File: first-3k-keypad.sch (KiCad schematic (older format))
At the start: 14 parts

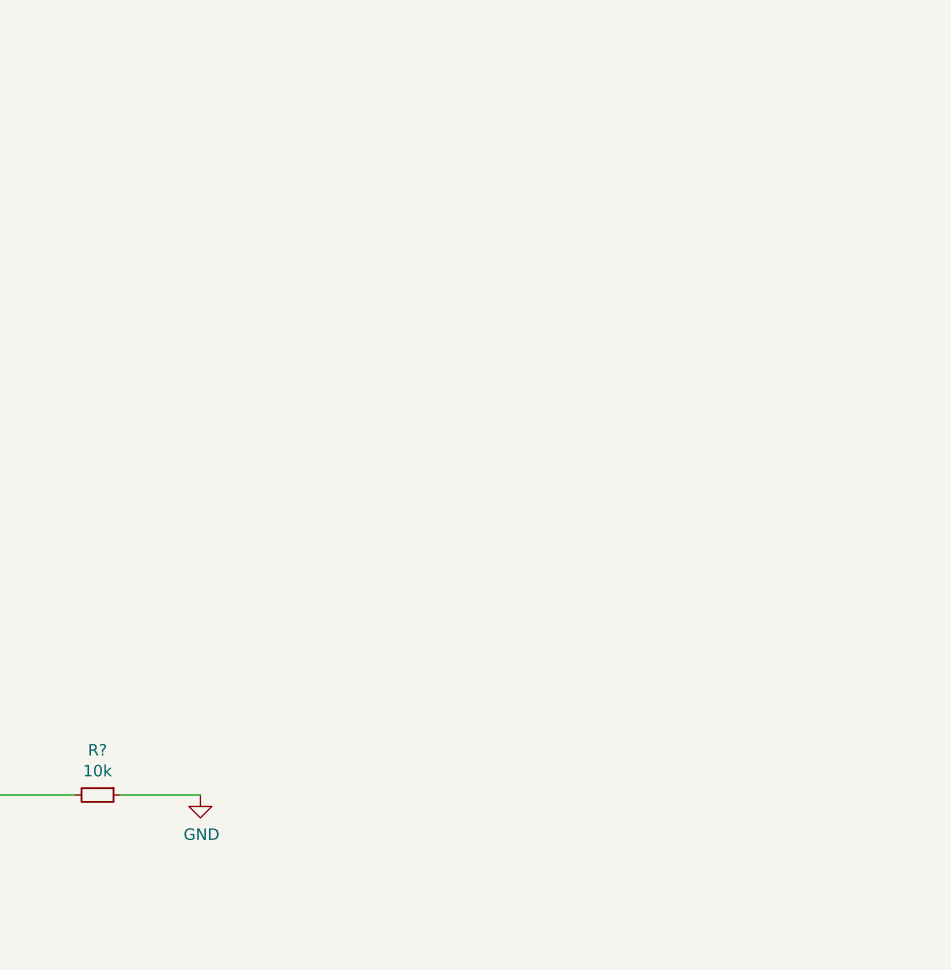
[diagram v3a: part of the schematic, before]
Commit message: Finished Schematic
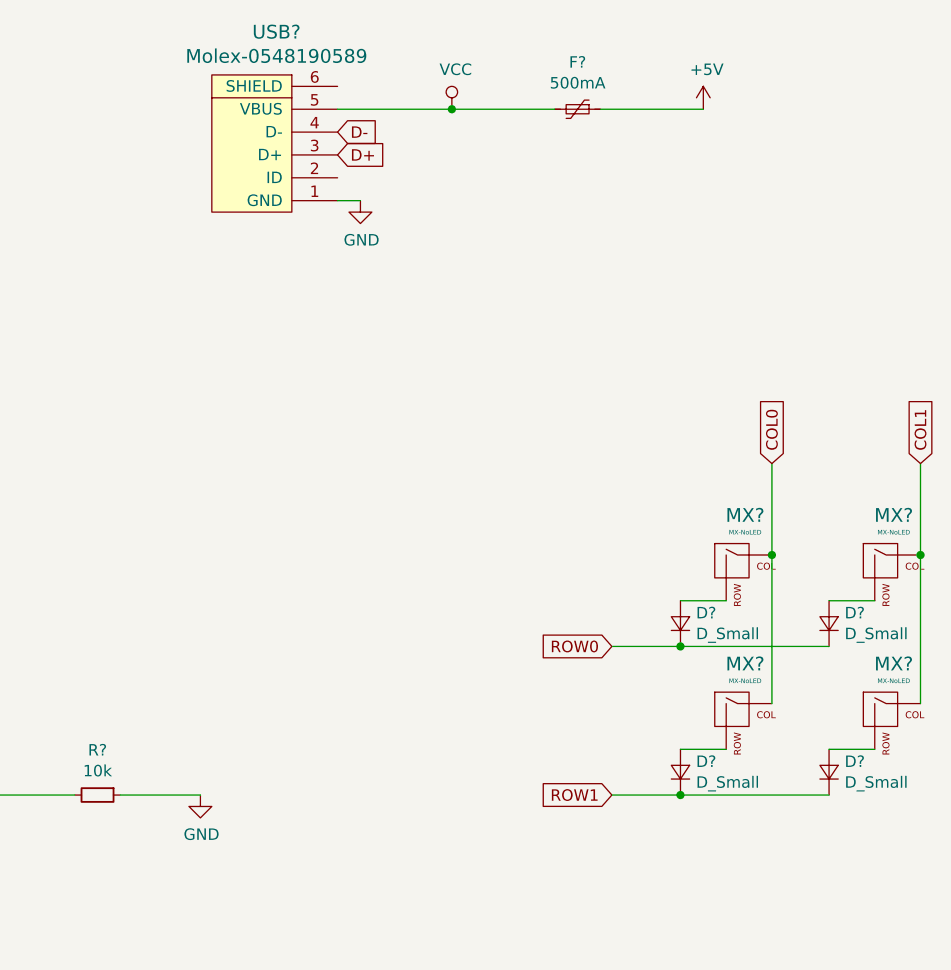
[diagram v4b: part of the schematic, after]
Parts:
- added D? (x4): D_Small, symbol Device:D_Small
- added F?: 500mA, symbol Device:Polyfuse_Small
- added MX? (x4): MX-NoLED, symbol MX_Alps_Hybrid:MX-NoLED
- added USB?: Molex-0548190589, symbol random-keyboard-parts:Molex-0548190589
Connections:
- net +5V: now also F?.1
- net D+: now also USB?.3 (D+)
- net D-: now also USB?.4 (D-)
- net GND: now also USB?.1 (GND)
- new net: D?.2 (A), MX?.2 (ROW) (x4)
- new net COL0: MX?.1 (COL), MX?.1 (COL)
- new net COL1: MX?.1 (COL), MX?.1 (COL)
- new net ROW0: D?.1 (K), D?.1 (K)
- new net ROW1: D?.1 (K), D?.1 (K)
- new net VCC: F?.2, USB?.5 (VBUS)
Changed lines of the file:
@@
 Text GLabel 4000 3500 0    50   Input ~ 0
 D-
+$Comp
+L random-keyboard-parts:Molex-0548190589 USB?
+U 1 1 6353D7B6
+P 7900 1700
+F 0 "USB?" V 8437 1667 60  0000 C CNN
+F 1 "Molex-0548190589" V 8331 1667 60  0000 C CNN
+F 2 "" H 7900 1700 60  0001 C CNN
+F 3 "" H 7900 1700 60  0001 C CNN
+	1    7900 1700
+	0    -1   -1   0
+$EndComp
+$Comp
+L Device:Polyfuse_Small F?
+U 1 1 6353F2F1
+P 9250 1500
+F 0 "F?" V 9045 1500 50  0000 C CNN
+F 1 "500mA" V 9136 1500 50  0000 C CNN
+F 2 "" H 9300 1300 50  0001 L CNN
+F 3 "~" H 9250 1500 50  0001 C CNN
+	1    9250 1500
+	0    1    1    0
+$EndComp
+$Comp
+L power:+5V #PWR?
+U 1 1 63542566
+P 9800 1500
+F 0 "#PWR?" H 9800 1350 50  0001 C CNN
+F 1 "+5V" H 9815 1673 50  0000 C CNN
+F 2 "" H 9800 1500 50  0001 C CNN
+F 3 "" H 9800 1500 50  0001 C CNN
+	1    9800 1500
+	1    0    0    -1
+$EndComp
+Wire Wire Line
+	9800 1500 9350 1500
+$Comp
+L power:VCC #PWR?
+U 1 1 63543A2B
+P 8700 1500
+F 0 "#PWR?" H 8700 1350 50  0001 C CNN
+F 1 "VCC" H 8717 1673 50  0000 C CNN
+F 2 "" H 8700 1500 50  0001 C CNN
+F 3 "" H 8700 1500 50  0001 C CNN
+	1    8700 1500
+	1    0    0    -1
+$EndComp
+Wire Wire Line
+	8200 1500 8700 1500
+Connection ~ 8700 1500
+Wire Wire Line
+	8700 1500 9150 1500
+Text GLabel 8200 1600 2    50   Input ~ 0
+D-
+Text GLabel 8200 1700 2    50   Input ~ 0
+D+
+$Comp
+L power:GND #PWR?
+U 1 1 63546D0F
+P 8300 1900
+F 0 "#PWR?" H 8300 1650 50  0001 C CNN
+F 1 "GND" H 8305 1727 50  0000 C CNN
+F 2 "" H 8300 1900 50  0001 C CNN
+F 3 "" H 8300 1900 50  0001 C CNN
+	1    8300 1900
+	1    0    0    -1
+$EndComp
+Wire Wire Line
+	8300 1900 8200 1900
+$Comp
+L MX_Alps_Hybrid:MX-NoLED MX?
+U 1 1 63548E84
+P 9950 3500
+F 0 "MX?" H 9983 3723 60  0000 C CNN
+F 1 "MX-NoLED" H 9983 3649 20  0000 C CNN
+F 2 "" H 9325 3475 60  0001 C CNN
+F 3 "" H 9325 3475 60  0001 C CNN
+	1    9950 3500
+	1    0    0    -1
+$EndComp
+$Comp
+L Device:D_Small D?
+U 1 1 6354A380
+P 9700 3750
+F 0 "D?" V 9746 3682 50  0000 R CNN
+F 1 "D_Small" V 9655 3682 50  0000 R CNN
+F 2 "" V 9700 3750 50  0001 C CNN
+F 3 "~" V 9700 3750 50  0001 C CNN
+	1    9700 3750
+	0    -1   -1   0
+$EndComp
+Wire Wire Line
+	9700 3650 9900 3650
+$Comp
+L MX_Alps_Hybrid:MX-NoLED MX?
+U 1 1 63552C0D
+P 10600 3500
+F 0 "MX?" H 10633 3723 60  0000 C CNN
+F 1 "MX-NoLED" H 10633 3649 20  0000 C CNN
+F 2 "" H 9975 3475 60  0001 C CNN
+F 3 "" H 9975 3475 60  0001 C CNN
+	1    10600 3500
+	1    0    0    -1
+$EndComp
+$Comp
+L Device:D_Small D?
+U 1 1 63552C17
+P 10350 3750
+F 0 "D?" V 10396 3682 50  0000 R CNN
+F 1 "D_Small" V 10305 3682 50  0000 R CNN
+F 2 "" V 10350 3750 50  0001 C CNN
+F 3 "~" V 10350 3750 50  0001 C CNN
+	1    10350 3750
+	0    -1   -1   0
+$EndComp
+Wire Wire Line
+	10350 3650 10550 3650
+$Comp
+L MX_Alps_Hybrid:MX-NoLED MX?
+U 1 1 63556D1C
+P 9950 4150
+F 0 "MX?" H 9983 4373 60  0000 C CNN
+F 1 "MX-NoLED" H 9983 4299 20  0000 C CNN
+F 2 "" H 9325 4125 60  0001 C CNN
+F 3 "" H 9325 4125 60  0001 C CNN
+	1    9950 4150
+	1    0    0    -1
+$EndComp
+$Comp
+L Device:D_Small D?
+U 1 1 63556D26
+P 9700 4400
+F 0 "D?" V 9746 4332 50  0000 R CNN
+F 1 "D_Small" V 9655 4332 50  0000 R CNN
+F 2 "" V 9700 4400 50  0001 C CNN
+F 3 "~" V 9700 4400 50  0001 C CNN
+	1    9700 4400
+	0    -1   -1   0
+$EndComp
+Wire Wire Line
+	9700 4300 9900 4300
+$Comp
+L MX_Alps_Hybrid:MX-NoLED MX?
+U 1 1 63559CA6
+P 10600 4150
+F 0 "MX?" H 10633 4373 60  0000 C CNN
+F 1 "MX-NoLED" H 10633 4299 20  0000 C CNN
+F 2 "" H 9975 4125 60  0001 C CNN
+F 3 "" H 9975 4125 60  0001 C CNN
+	1    10600 4150
+	1    0    0    -1
+$EndComp
+$Comp
+L Device:D_Small D?
+U 1 1 63559CB0
+P 10350 4400
+F 0 "D?" V 10396 4332 50  0000 R CNN
+F 1 "D_Small" V 10305 4332 50  0000 R CNN
+F 2 "" V 10350 4400 50  0001 C CNN
+F 3 "~" V 10350 4400 50  0001 C CNN
+	1    10350 4400
+	0    -1   -1   0
+$EndComp
+Wire Wire Line
+	10350 4300 10550 4300
+Wire Wire Line
+	10100 3050 10100 3450
+Connection ~ 10100 3450
+Wire Wire Line
+	10100 3450 10100 4100
+Wire Wire Line
+	10750 3050 10750 3450
+Connection ~ 10750 3450
+Wire Wire Line
+	10750 3450 10750 4100
+Wire Wire Line
+	10350 3850 9700 3850
+Connection ~ 9700 3850
+Wire Wire Line
+	9700 3850 9400 3850
+Wire Wire Line
+	10350 4500 9700 4500
+Connection ~ 9700 4500
+Wire Wire Line
+	9700 4500 9400 4500
+Text GLabel 9400 3850 0    50   Input ~ 0
+ROW0
+Text GLabel 9400 4500 0    50   Input ~ 0
+ROW1
+Text GLabel 10100 3050 1    50   Input ~ 0
+COL0
+Text GLabel 10750 3050 1    50   Input ~ 0
+COL1
 $EndSCHEMATC
